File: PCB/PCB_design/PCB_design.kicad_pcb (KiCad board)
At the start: 2 copper layers, 117 x 56.8 mm, 49 parts, among them J2 Conn_01x03_Pin, J3 Conn_01x01_Pin, J4 Conn_01x01_Pin, J5 Conn_01x01_Pin, J6 Conn_01x01_Pin, J7 Conn_02x04_Counter_Clockwise, K1 Relay_SPST-NO, K2 Relay_SPST-NO, K3 Relay_SPST-NO, K4 Relay_SPST-NO, Q1 MMBT3904, Q2 MMBT3904, Q3 MMBT3904, Q4 MMBT3904, T1 Transformer_1P_2S, U1 SCJT1117B-3.3-A

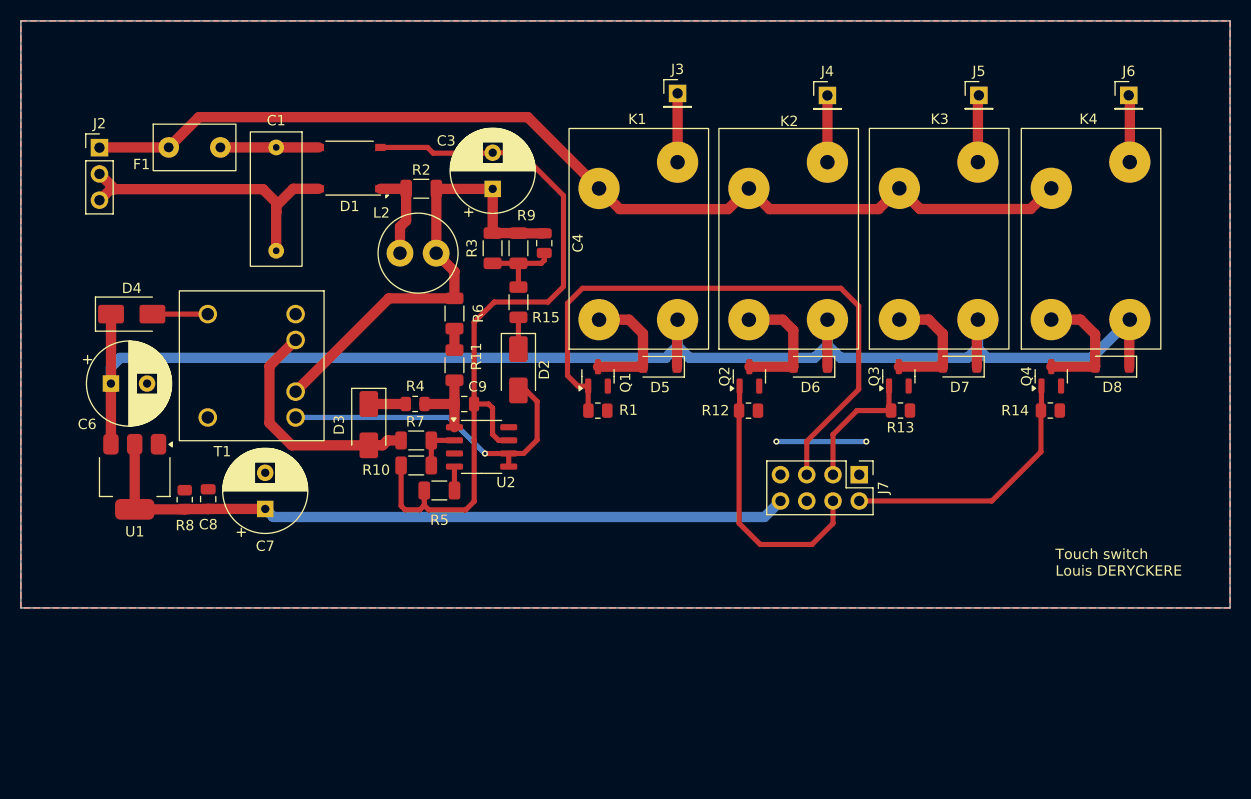
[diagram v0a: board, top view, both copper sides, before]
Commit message: Routage compact
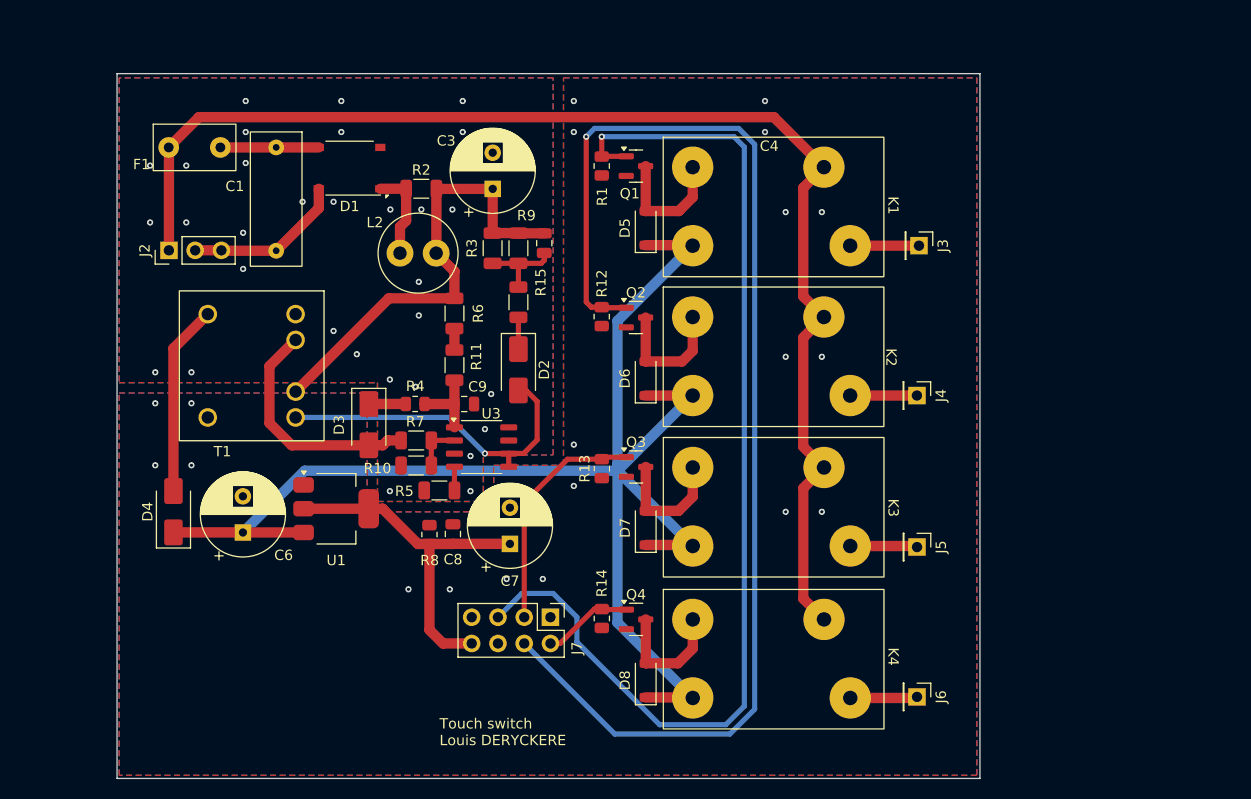
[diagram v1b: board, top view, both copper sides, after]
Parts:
- removed U2: ~, Package_SO:SOP-8_3.9x4.9mm_P1.27mm
- added U3: ~, Package_SO:SOP-8_3.9x4.9mm_P1.27mm, F.Cu at (113.6, 61.2)
- moved J6 61.7 mm to (155.7, 85.4), turned to -90 degrees
- moved K4 55.9 mm to (134.0, 85.5), turned to 0 degrees
- moved D8 54.4 mm to (129.5, 83.8), turned to 90 degrees
- moved R14 47.8 mm to (125.2, 77.8), turned to 90 degrees
- moved Q4 46.6 mm to (128.5, 77.9), turned to 0 degrees
- moved J5 44.1 mm to (155.7, 70.9), turned to -90 degrees
- moved K3 35.2 mm to (134.0, 70.8), turned to 0 degrees
- moved D7 34.2 mm to (129.5, 69.1), turned to 90 degrees
- moved J7 32.9 mm to (120.2, 77.7)
- moved J4 30.3 mm to (155.7, 56.2), turned to -90 degrees
- moved R13 29.4 mm to (125.2, 63.3), turned to 90 degrees
- moved J3 27.6 mm to (155.9, 41.8), turned to -90 degrees
- moved Q3 26.9 mm to (128.5, 63.2), turned to 0 degrees
- moved R8 23.9 mm to (108.5, 69.7)
- moved C8 23.9 mm to (110.8, 69.7)
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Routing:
- net CT2: track 26.2 -> 118.9 mm, vias 0 -> 1
- net GND: track 75.5 -> 0.00 mm, vias 0 -> 31
- net CT1: track 59.7 -> 104.8 mm, vias 0 -> 1
- net +3.3V: track 69.8 -> 34.3 mm
- net L: track 101.2 -> 125.3 mm
- net CT4: track 25.9 -> 8.75 mm
- net N: track 30.3 -> 15.6 mm
- net Net-(D4-A): track 5.36 -> 18.5 mm
- net CT3: track 12.9 -> 22.8 mm
- net GND2: track 8.70 -> 0.00 mm, vias 2 -> 20
- net +5VDC: track 146.6 -> 140.6 mm
- added copper zone on B.Cu, net GND2
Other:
- board size 117 x 56.8 mm -> 83.5 x 68.2 mm
